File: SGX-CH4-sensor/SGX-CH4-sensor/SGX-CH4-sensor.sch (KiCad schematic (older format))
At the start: 3 parts

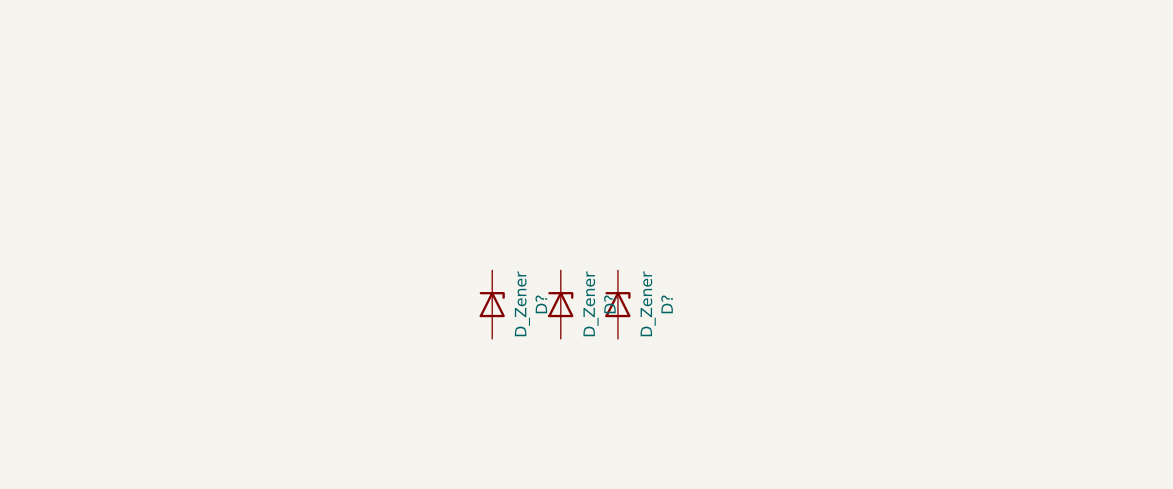
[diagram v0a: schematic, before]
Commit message: fewf
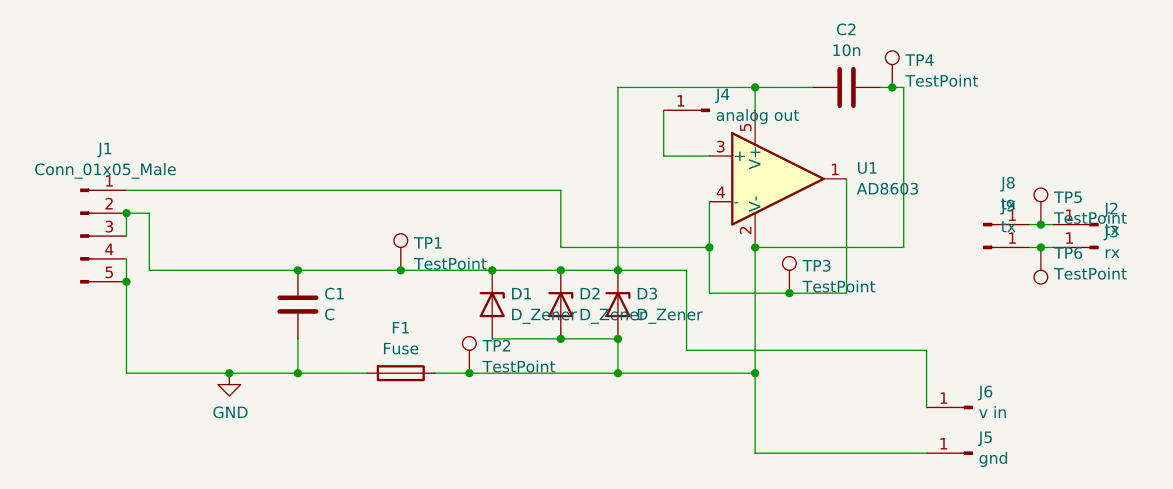
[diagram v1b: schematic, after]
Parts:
- removed D? (x2): D_Zener, symbol Device:D_Zener
- added C1: C, Capacitor_THT:CP_Radial_D8.0mm_P5.00mm, symbol Device:C
- added C2: 10n, Capacitor_THT:CP_Radial_D6.3mm_P2.50mm, symbol Device:C
- added D1, D2: D_Zener, Diode_THT:D_DO-35_SOD27_P10.16mm_Horizontal, symbol Device:D_Zener
- added F1: Fuse, Resistor_THT:R_Axial_DIN0309_L9.0mm_D3.2mm_P5.08mm_Vertical, symbol Device:Fuse
- added J1: Conn_01x05_Male, Connector_PinHeader_2.54mm:PinHeader_1x05_P2.54mm_Vertical, symbol Connector:Conn_01x05_Male
- added J2, J8, J9: tx, Connector_PinHeader_2.54mm:PinHeader_1x01_P2.54mm_Vertical, symbol Connector:Conn_01x01_Male
- added J3: rx, Connector_PinHeader_2.54mm:PinHeader_1x01_P2.54mm_Vertical, symbol Connector:Conn_01x01_Male
- added J4: analog out, Connector_PinHeader_2.54mm:PinHeader_1x01_P2.54mm_Vertical, symbol Connector:Conn_01x01_Male
- added J5: gnd, Connector_PinHeader_2.54mm:PinHeader_1x01_P2.54mm_Vertical, symbol Connector:Conn_01x01_Male
- added J6: v in, Connector_PinHeader_2.54mm:PinHeader_1x01_P2.54mm_Vertical, symbol Connector:Conn_01x01_Male
- added TP1, TP2, TP3, TP4, TP5, TP6: TestPoint, TestPoint:TestPoint_Pad_D3.0mm, symbol Connector:TestPoint
- added U1: AD8603, Package_TO_SOT_SMD:SOT-23-5, symbol Amplifier_Operational:AD8603
- D3: renamed from D?; footprint (none) -> Diode_THT:D_DO-35_SOD27_P10.16mm_Horizontal
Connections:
- net at D3.1 (K): now also C1.1, C2.1, D1.1 (K), D2.1 (K), J1.2 (Pin_2), J1.3 (Pin_3), J6.1 (Pin_1), TP1.1, U1.5 (V+)
- net at D3.2 (A): now also C2.2, D1.2 (A), D2.2 (A), F1.1, J5.1 (Pin_1), TP2.1, TP4.1, U1.2 (V-)
- new net: J2.1 (Pin_1), J8.1 (Pin_1), TP5.1
- new net: J3.1 (Pin_1), J9.1 (Pin_1), TP6.1
- new net: J4.1 (Pin_1), U1.3 (+)
- new net: J1.1 (Pin_1), TP3.1, U1.1, U1.4 (-)
- new net GND: C1.2, F1.2, J1.4 (Pin_4), J1.5 (Pin_5)
